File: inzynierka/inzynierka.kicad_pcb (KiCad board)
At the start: 2 copper layers, 95.8 x 52 mm, 107 parts, among them J101 Conn_01x10, Q501 Q_PNP_BCE, Q502 BC848, T501 Transformer_1P_1S, U101 LM1117-3.3, U102 MCP6L04x-xSL, U103 LM239D, U201 SPU0410LR5H-QB, U202 MCP6L04x-xSL, U301 SPU0410LR5H-QB, U302 MCP6L04x-xSL, U401 SPU0410LR5H-QB, U402 MCP6L04x-xSL

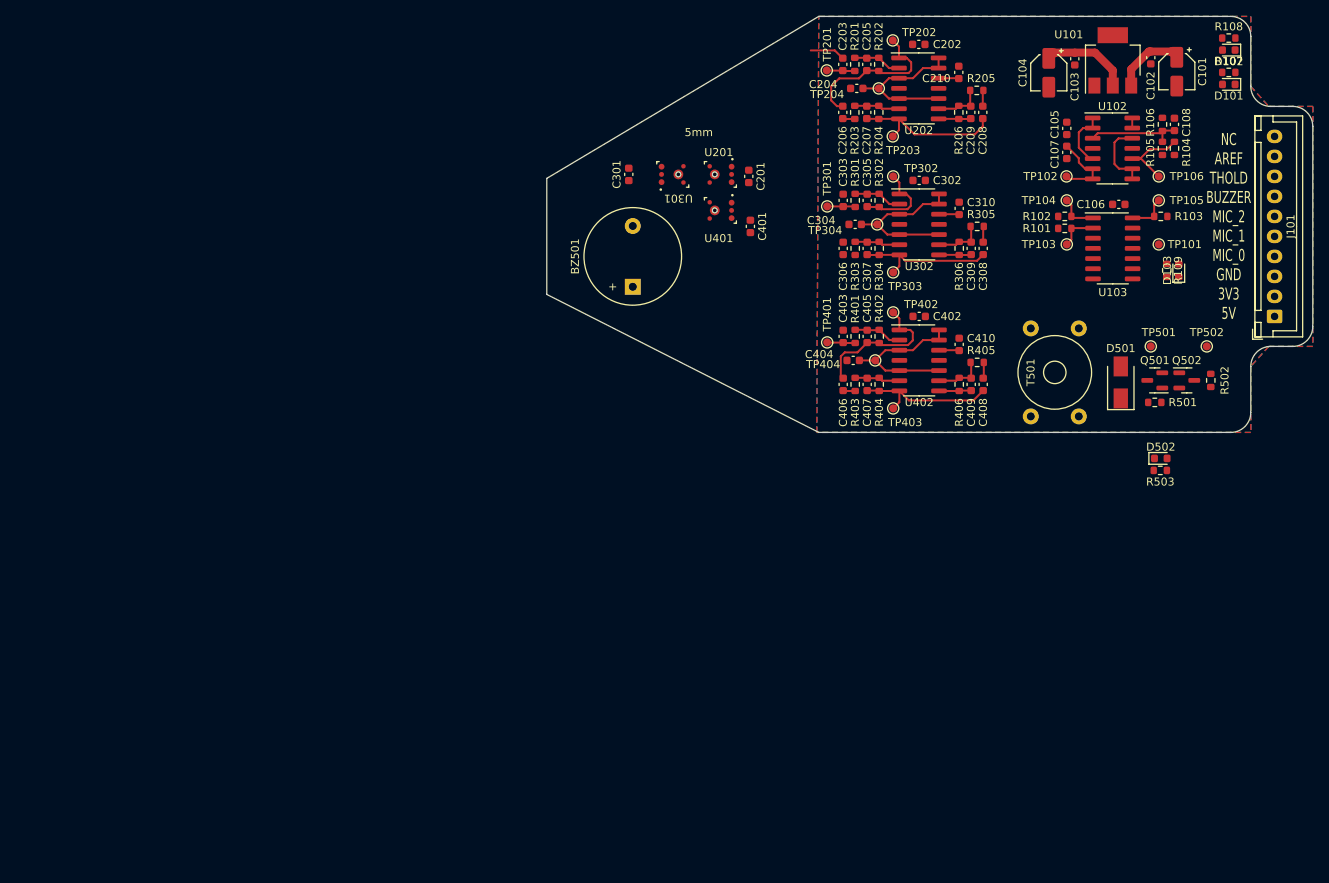
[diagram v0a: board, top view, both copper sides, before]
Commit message: shield shape
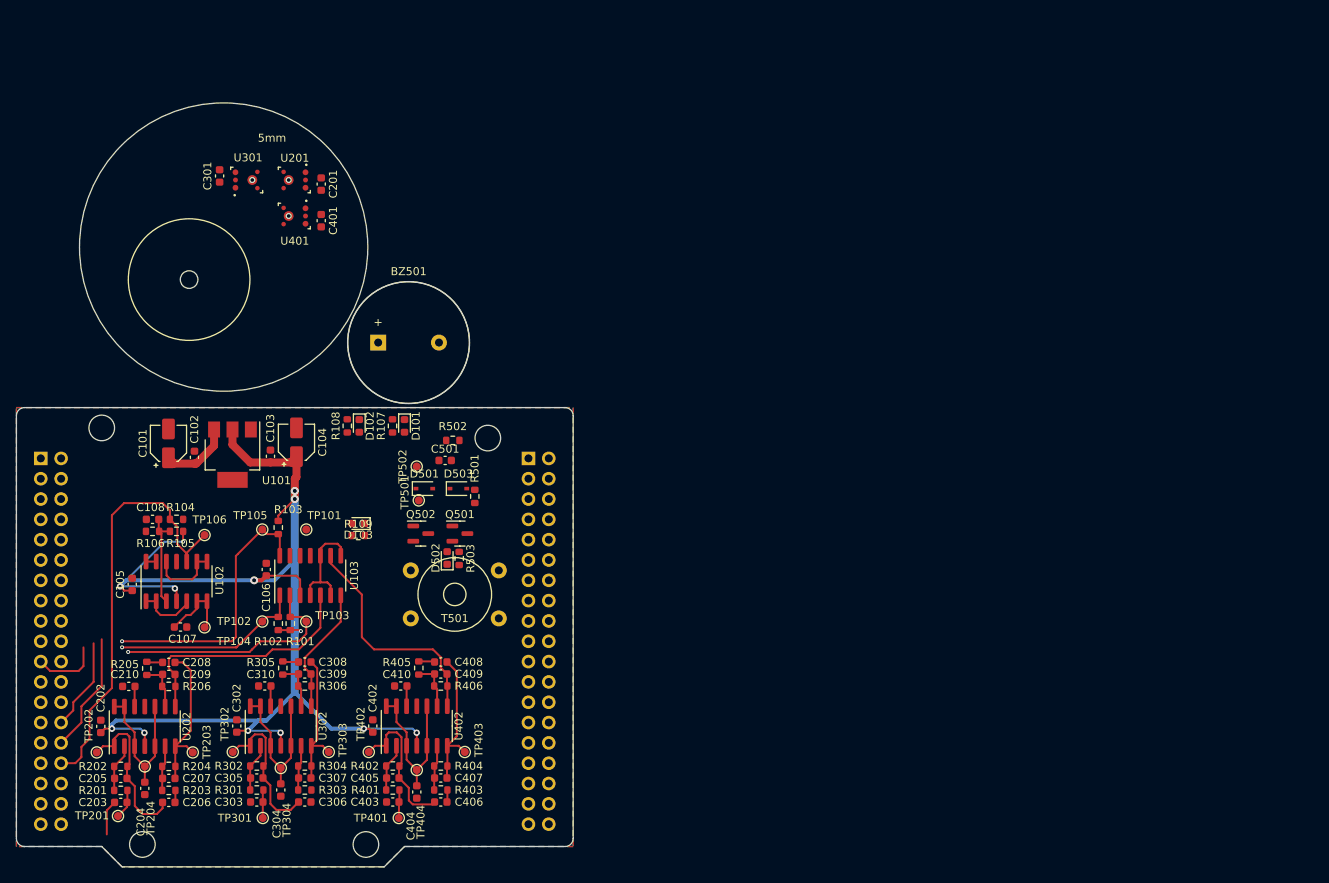
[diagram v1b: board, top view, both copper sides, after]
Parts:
- added C501: C_Small, Capacitor_SMD:C_0603_1608Metric, F.Cu at (124.8, 86.5)
- added D503: 1N5819WS, Diode_SMD:D_SOD-323, F.Cu at (126.4, 90.0)
- added H101: MountingHole, MountingHole:MountingHole_3.2mm_M3, F.Cu at (114.9, 134.5)
- added H102: MountingHole, MountingHole:MountingHole_3.2mm_M3, F.Cu at (87.0, 134.5)
- added H103: MountingHole, MountingHole:MountingHole_3.2mm_M3, F.Cu at (130.1, 83.7)
- added H104: MountingHole, MountingHole:MountingHole_3.2mm_M3, F.Cu at (81.9, 82.4)
- added H501: BuzzerHole, MountingHole:MountingHole_2.2mm_M2, F.Cu at (92.8, 63.9)
- added J102: SHIELD_RIGHT, Connector_PinSocket_2.54mm:PinSocket_2x19_P2.54mm_Vertical, B.Cu at (135.2, 86.2)
- BZ501: footprint Buzzer_Beeper:Buzzer_12x9.5RM7.6 -> Buzzer_Beeper:Buzzer_15x7.5RM7.6
- D501: value US1M -> 1N5819WS; footprint Diode_SMD:D_SMA -> Diode_SMD:D_SOD-323
- J101: value Conn_01x10 -> SHIELD_LEFT; footprint Connector_JST:JST_XH_B10B-XH-A_1x10_P2.50mm_Vertical -> Connector_PinSocket_2.54mm:PinSocket_2x19_P2.54mm_Vertical; moved to B.Cu
- Q501: value Q_PNP_BCE -> SS8550
- Q502: value BC848 -> MMBT3904
- moved J101 155.2 mm to (74.2, 86.2), turned to 180 degrees
- moved C108 136.9 mm to (88.2, 93.9), turned to 180 degrees
- moved R106 136.1 mm to (88.2, 95.4), turned to 180 degrees
- moved C101 134.3 mm to (90.2, 84.4), turned to 90 degrees
- moved TP202 133.5 mm to (81.2, 123.0), turned to 90 degrees
- moved C202 133.1 mm to (81.8, 119.8), turned to 90 degrees
- moved R104 133.1 mm to (91.2, 93.9), turned to 0 degrees
- moved R105 132.2 mm to (91.2, 95.4), turned to 180 degrees
- moved C105 130.0 mm to (85.7, 102.0)
- moved C102 129.6 mm to (93.5, 86.1), turned to 90 degrees
- moved R202 129.1 mm to (84.2, 124.8), turned to 0 degrees
- moved C205 129.1 mm to (84.2, 126.2), turned to 0 degrees
- moved C203 129.1 mm to (84.2, 129.2), turned to 0 degrees
- moved C210 129.1 mm to (85.2, 114.8), turned to 180 degrees
- moved R201 129.0 mm to (84.2, 127.8), turned to 180 degrees
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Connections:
- BZ501 pad 1: Net-(BZ501-Pad1) -> Net-(T501-Pad1)
- BZ501 pad 2: Net-(BZ501-Pad2) -> Net-(T501-Pad2)
- C105 pad 2: GND -> GNDA
- C107 pad 2: GND -> GNDA
- C108 pad 2: GND -> GNDA
- C201 pad 2: GND -> GNDA
- C202 pad 2: GND -> GNDA
- C204 pad 1: GND -> GNDA
- C210 pad 2: GND -> GNDA
- C301 pad 2: GND -> GNDA
- C302 pad 2: GND -> GNDA
- C304 pad 1: GND -> GNDA
- C310 pad 2: GND -> GNDA
- C401 pad 2: GND -> GNDA
- C402 pad 2: GND -> GNDA
- C404 pad 1: GND -> GNDA
- C410 pad 2: GND -> GNDA
- D501 pad 1: Net-(D501-Pad1) -> Net-(Q501-Pad3)
- J101 pad 1: +5V -> unconnected-(J101-Pad1)
- J101 pad 2: +3V3 -> unconnected-(J101-Pad2)
- J101 pad 3: GND -> unconnected-(J101-Pad3)
- J101 pad 4: OUT_0 -> unconnected-(J101-Pad4)
- J101 pad 5: OUT_1 -> unconnected-(J101-Pad5)
- J101 pad 6: OUT_2 -> unconnected-(J101-Pad6)
- J101 pad 7: PIEZO -> unconnected-(J101-Pad7)
- J101 pad 8: THRESHOLD_MCU -> GND
- J101 pad 9: AREF -> unconnected-(J101-Pad9)
- Q501 pad 2: Net-(D501-Pad1) -> +5V
- Q501 pad 3: +3V3 -> Net-(Q501-Pad3)
- R104 pad 2: GND -> GNDA
- R106 pad 2: GND -> GNDA
- R502 pad 2: PIEZO -> Net-(R502-Pad2)
- R503 pad 1: Net-(D501-Pad1) -> Net-(Q501-Pad3)
- T501 pad 1: Net-(BZ501-Pad2) -> Net-(T501-Pad1)
- T501 pad 2: Net-(BZ501-Pad1) -> Net-(T501-Pad2)
- T501 pad 4: Net-(D501-Pad1) -> Net-(Q501-Pad3)
- TP501 pad 1: Net-(D501-Pad1) -> Net-(Q501-Pad3)
- TP502 pad 1: PIEZO -> /TRANSMITER/PIEZO_IN
- U102 pad 11: GND -> GNDA
- U201 pad 2: GND -> GNDA
- U201 pad 3: GND -> GNDA
- U201 pad 5: GND -> GNDA
- U201 pad 6: GND -> GNDA
- U202 pad 11: GND -> GNDA
- U301 pad 2: GND -> GNDA
- U301 pad 3: GND -> GNDA
- U301 pad 5: GND -> GNDA
- U301 pad 6: GND -> GNDA
- U302 pad 11: GND -> GNDA
- U401 pad 2: GND -> GNDA
- U401 pad 3: GND -> GNDA
- U401 pad 5: GND -> GNDA
- U401 pad 6: GND -> GNDA
- U402 pad 11: GND -> GNDA
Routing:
- net +3V3: track 11.1 -> 164.1 mm, vias 0 -> 13
- net THRESHOLD_MCU: track 10.4 -> 54.4 mm
- net OUT_2: track 5.02 -> 42.7 mm, vias 0 -> 1
- net OUT_0: track 4.95 -> 41.3 mm, vias 0 -> 1
- net OUT_1: track 5.02 -> 38.9 mm, vias 0 -> 1
- net MIC_0: track 4.05 -> 31.0 mm
- net MIC_2: track 4.05 -> 29.2 mm
- net THRESHOLD_OP: track 1.27 -> 14.9 mm
- net MIC_1: track 4.05 -> 16.1 mm
- net Net-(C305-Pad2): track 10.9 -> 18.7 mm
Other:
- board size 95.8 x 52 mm -> 69.6 x 95.5 mm
- board text removed: "NC AREF THOLD BUZZER MIC_2 MIC_1 MIC_0 GND 3V3 5V"
